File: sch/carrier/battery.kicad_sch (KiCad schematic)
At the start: 9 parts

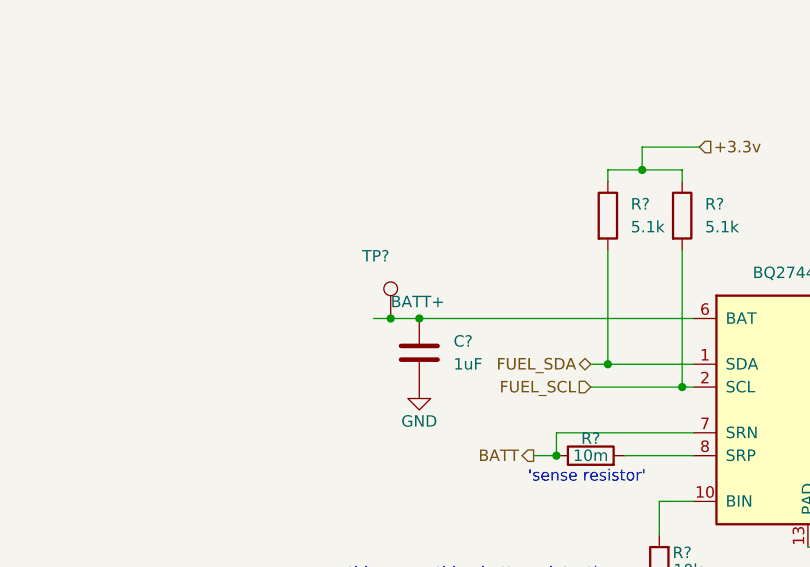
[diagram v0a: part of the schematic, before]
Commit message: push updates
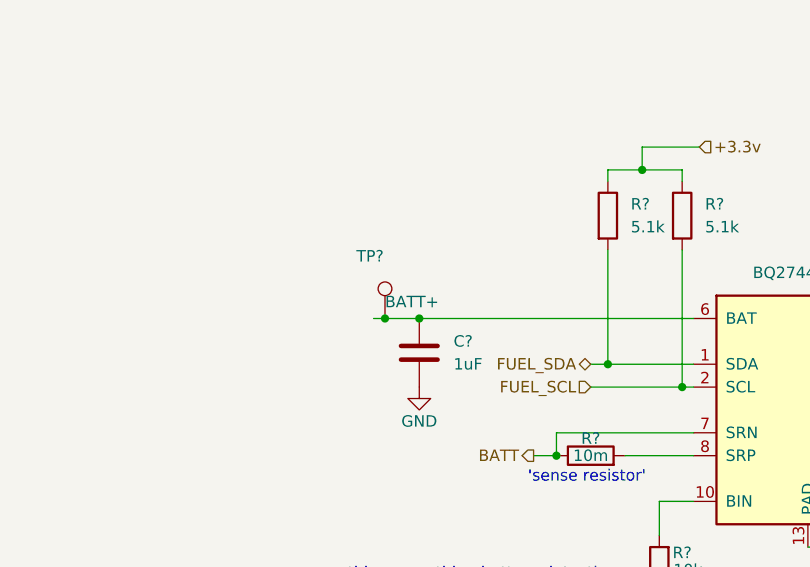
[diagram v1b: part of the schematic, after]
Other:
- moved on the sheet: TP?
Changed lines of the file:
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@@
     (comment 1 "https://www.github.com/cinnamondev/gamepithing")
   )
-  (junction (at 92.71 72.39) (diameter 0.9144) (color 0 0 0 0))
+  (junction (at 92.075 72.39) (diameter 0.9144) (color 0 0 0 0))
   (junction (at 95.885 72.39) (diameter 0.9144) (color 0 0 0 0))
   (junction (at 111.125 87.63) (diameter 0.9144) (color 0 0 0 0))
@@
   (junction (at 158.75 74.93) (diameter 0.9144) (color 0 0 0 0))
   (no_connect (at 146.05 5.715))
-  (wire (pts (xy 90.805 72.39) (xy 92.71 72.39))
+  (wire (pts (xy 90.805 72.39) (xy 92.075 72.39))
     (stroke (width 0) (type solid) (color 0 0 0 0))
   )
-  (wire (pts (xy 92.71 72.39) (xy 95.885 72.39))
+  (wire (pts (xy 92.075 72.39) (xy 95.885 72.39))
     (stroke (width 0) (type solid) (color 0 0 0 0))
   )
@@
     (effects (font (size 1.27 1.27)) (justify left))
   )
-  (symbol (lib_id "Connector:TestPoint") (at 92.71 72.39 0) (unit 1)
+  (symbol (lib_id "Connector:TestPoint") (at 92.075 72.39 0) (unit 1)
     (in_bom yes) (on_board yes)
-    (property "Reference" "TP?" (id 0) (at 89.535 65.4684 0)
+    (property "Reference" "TP?" (id 0) (at 88.9 65.4684 0)
       (effects (font (size 1.27 1.27)) (justify left))
     )
-    (property "Value" "BATT+" (id 1) (at 92.71 70.5484 0)
+    (property "Value" "BATT+" (id 1) (at 92.075 70.5484 0)
       (effects (font (size 1.27 1.27)) (justify left))
     )
-    (property "Footprint" "" (id 2) (at 97.79 72.39 0)
+    (property "Footprint" "" (id 2) (at 97.155 72.39 0)
       (effects (font (size 1.27 1.27)) hide)
     )
-    (property "Datasheet" "~" (id 3) (at 97.79 72.39 0)
+    (property "Datasheet" "~" (id 3) (at 97.155 72.39 0)
       (effects (font (size 1.27 1.27)) hide)
     )
